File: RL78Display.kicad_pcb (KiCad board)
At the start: 2 copper layers, 25.8 x 29.5 mm, 34 parts, among them J1 USB_B_Mini, J2 breadboardController, J3 TFT_ATM0130B3, Q1 Q_NMOS_GSD, SW1 SW_Push, SW2 SW_Push, U1 NJM2884U1, U2 RL78G13_64pin, Y1 32.768kHz

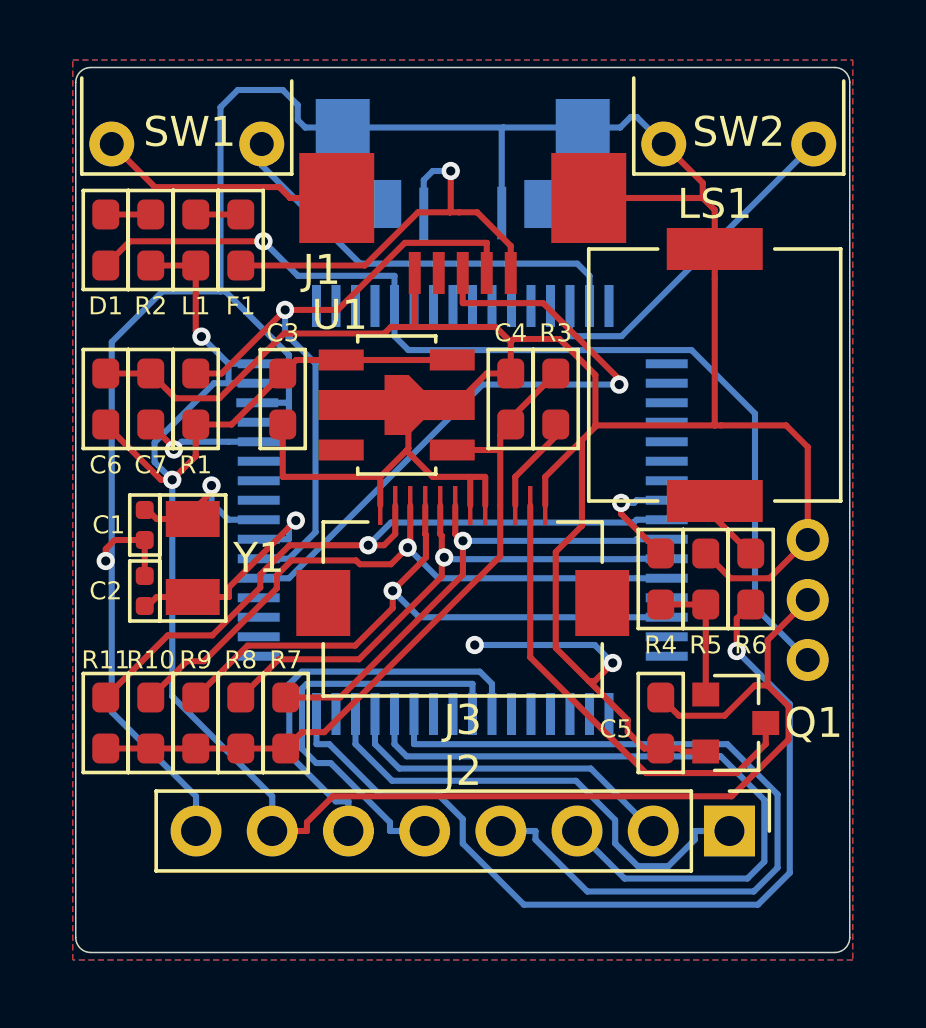
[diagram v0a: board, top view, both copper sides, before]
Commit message: 基板 V2.0
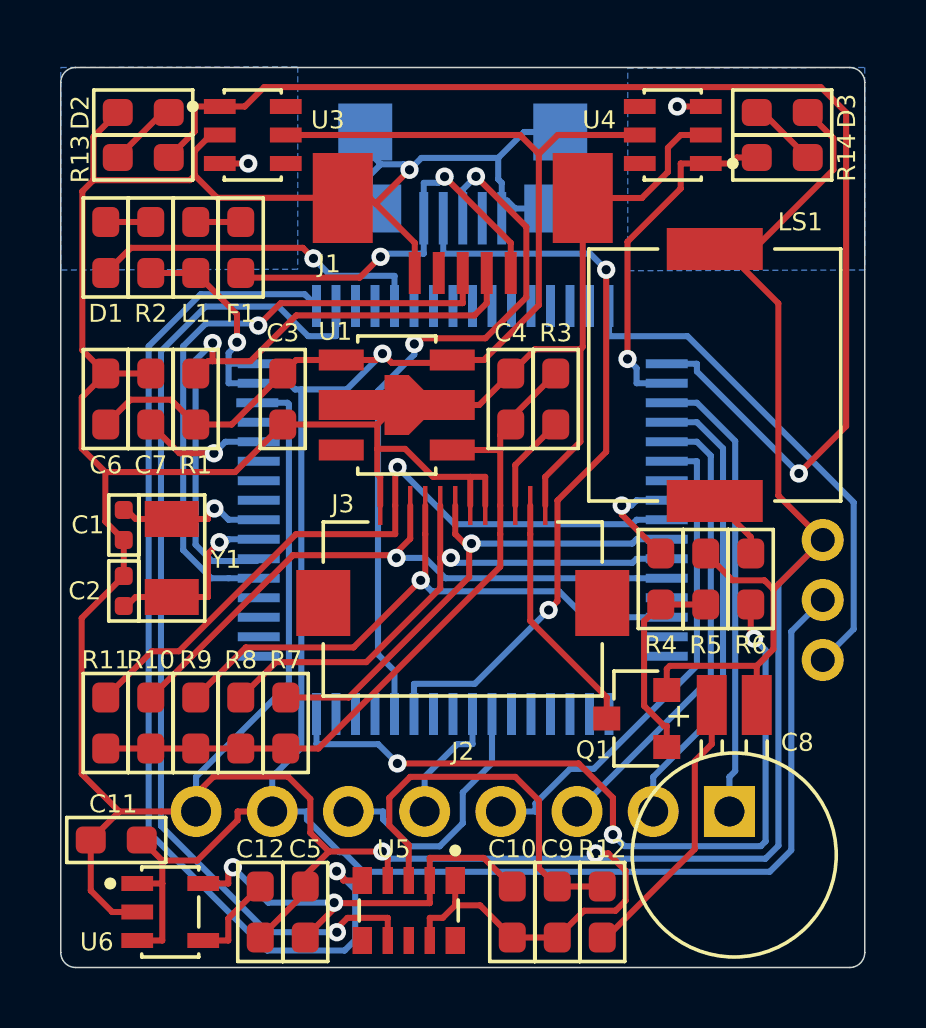
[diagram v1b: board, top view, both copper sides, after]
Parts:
- removed SW1, SW2: SW_Push, RL78Display:SW_THBP07-043C
- added C10: 0.1uF, RL78Display:1608Metric, F.Cu at (1.65, 13.4)
- added C11: 0.1uF, RL78Display:1608Metric, F.Cu at (-11.6, 11.0)
- added C12: 0.1uF, RL78Display:1608Metric, F.Cu at (-6.75, 13.4)
- added C8: 0.22F, RL78Display:DCK-3R3E224-E, F.Cu at (9.05, 11.5)
- added C9: 0.1uF, RL78Display:1608Metric, F.Cu at (3.15, 13.4)
- added D2: SW_L, RL78Display:1608Metric, F.Cu at (-10.7, -13.2)
- added D3: SW_R, RL78Display:1608Metric, F.Cu at (10.7, -13.2)
- added J4: USB_B_Micro, RL78Display:ZX62-B-5PA, B.Cu at (0.00, -12.6)
- added R12: 1k, RL78Display:1608Metric, F.Cu at (4.65, 13.4)
- added R13: R, RL78Display:1608Metric, F.Cu at (-10.7, -11.8)
- added R14: R, RL78Display:1608Metric, F.Cu at (10.7, -11.8)
- added U3: TTP223, RL78Display:SOT-23-6, F.Cu at (-7.00, -12.5)
- added U4: TTP223, RL78Display:SOT-23-6, F.Cu at (7.00, -12.5)
- added U5: RX8900CE, RL78Display:RX8900CE, F.Cu at (-1.80, 13.3)
- added U6: NJM2864, RL78Display:SOT-23-5, F.Cu at (-9.75, 13.4)
- C5: value 0.1uF -> 1uF
- J1: footprint RL78Display:Mini_Micro_USB_Connector -> RL78Display:UX60SC-MB-5ST
- moved C5 13.4 mm to (-5.25, 13.4), turned to 270 degrees
- moved Q1 3.30 mm to (5.80, 6.95), turned to 180 degrees
- moved C1 0.70 mm to (-11.3, 0.50)
- moved C2 0.70 mm to (-11.3, 2.70)
- moved Y1 0.70 mm to (-9.70, 1.60)
- moved J2 0.65 mm to (8.89, 10.1)
- moved TP1 0.50 mm to (12.0, 1.00)
- moved TP2 0.50 mm to (12.0, 3.00)
- moved TP3 0.50 mm to (12.0, 5.00)
- moved D1 0.25 mm to (-11.9, -8.75)
- moved F1 0.25 mm to (-7.40, -8.75)
- moved L1 0.25 mm to (-8.90, -8.75)
- moved R2 0.25 mm to (-10.4, -8.75)
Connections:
- C5 pad 2: +5V -> +3V0
- TP3 pad 1: LED_Status -> GPIO
- U2 pad 17: (no net) -> RTC_SCL
- U2 pad 18: (no net) -> RTC_SDA
- U2 pad 30: SW_R -> (no net)
- U2 pad 31: SW_L -> (no net)
- U2 pad 32: (no net) -> GPIO
- U2 pad 33: (no net) -> SW_L
- U2 pad 34: (no net) -> SW_R
- U2 pad 35: (no net) -> SW_A
- U2 pad 36: (no net) -> SW_B
- U2 pad 37: (no net) -> SW_C
- U2 pad 38: (no net) -> SW_D
- U2 pad 59: SW_D -> UART1_RX
- U2 pad 60: SW_C -> UART1_TX
- U2 pad 61: SW_B -> (no net)
- U2 pad 62: SW_A -> (no net)
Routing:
- net GND: track 166.2 -> 205.1 mm
- net RTC_SCL: track 0.00 -> 34.9 mm, vias 0 -> 1
- net RTC_SDA: track 0.00 -> 33.7 mm, vias 0 -> 1
- net +5V: track 68.7 -> 98.6 mm
- net SW_L: track 14.2 -> 43.1 mm, vias 0 -> 1
- net UART1_RX: track 0.00 -> 25.5 mm, vias 0 -> 2
- net UART1_TX: track 0.00 -> 23.7 mm, vias 0 -> 2
- net LED_Status: track 34.5 -> 11.4 mm
- net GPIO: track 0.00 -> 17.1 mm
- net +3V0: track 0.00 -> 14.7 mm, vias 0 -> 2
- net Net-(C9-Pad1): track 0.00 -> 13.2 mm
- net SW_D: track 26.8 -> 16.5 mm
- net POS_H: track 14.2 -> 4.21 mm
- net Net-(C8-Pad1): track 0.00 -> 9.34 mm
- net SW_C: track 23.3 -> 15.4 mm
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- added copper zone on B.Cu, net Net-(U3-Pad3)
- added copper zone on B.Cu, net Net-(U4-Pad3)
- removed copper zone on B.Cu, net GND
- removed copper zone on F.Cu, net GND
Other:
- board size 25.8 x 29.5 mm -> 26.8 x 30 mm
- board text added: "GPIO"
- board text added: "RL78 Display V2.0"
- board text removed: "RL78 Display V1.1"
- board text removed: "TP"
